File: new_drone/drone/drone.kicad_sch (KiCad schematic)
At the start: 29 parts, among them J1 Conn_01x06, SW1 SW_Push_Open, SW2 SW_Push_Open, U1 ESP32-WROOM-32, U2 MPU-6050, U4 BMP280, U5 MCP8063, U5 TPS63001, U6 MCP8063, U7 MCP8063, U8 MCP8063

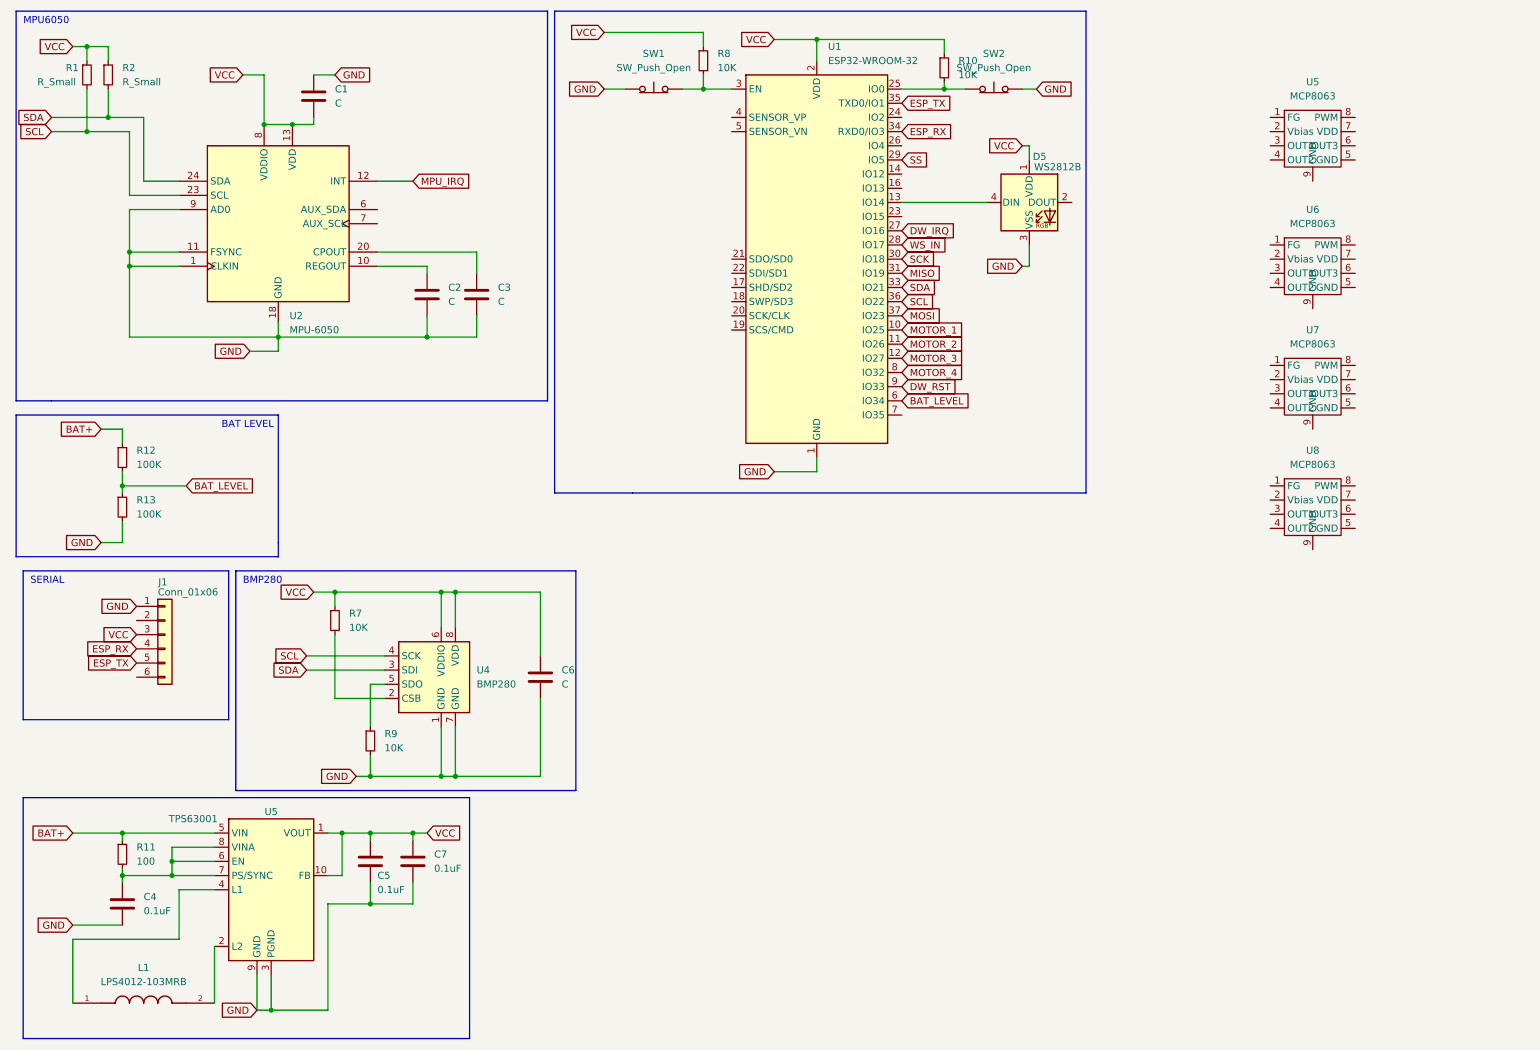
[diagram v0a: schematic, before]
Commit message: first wiring
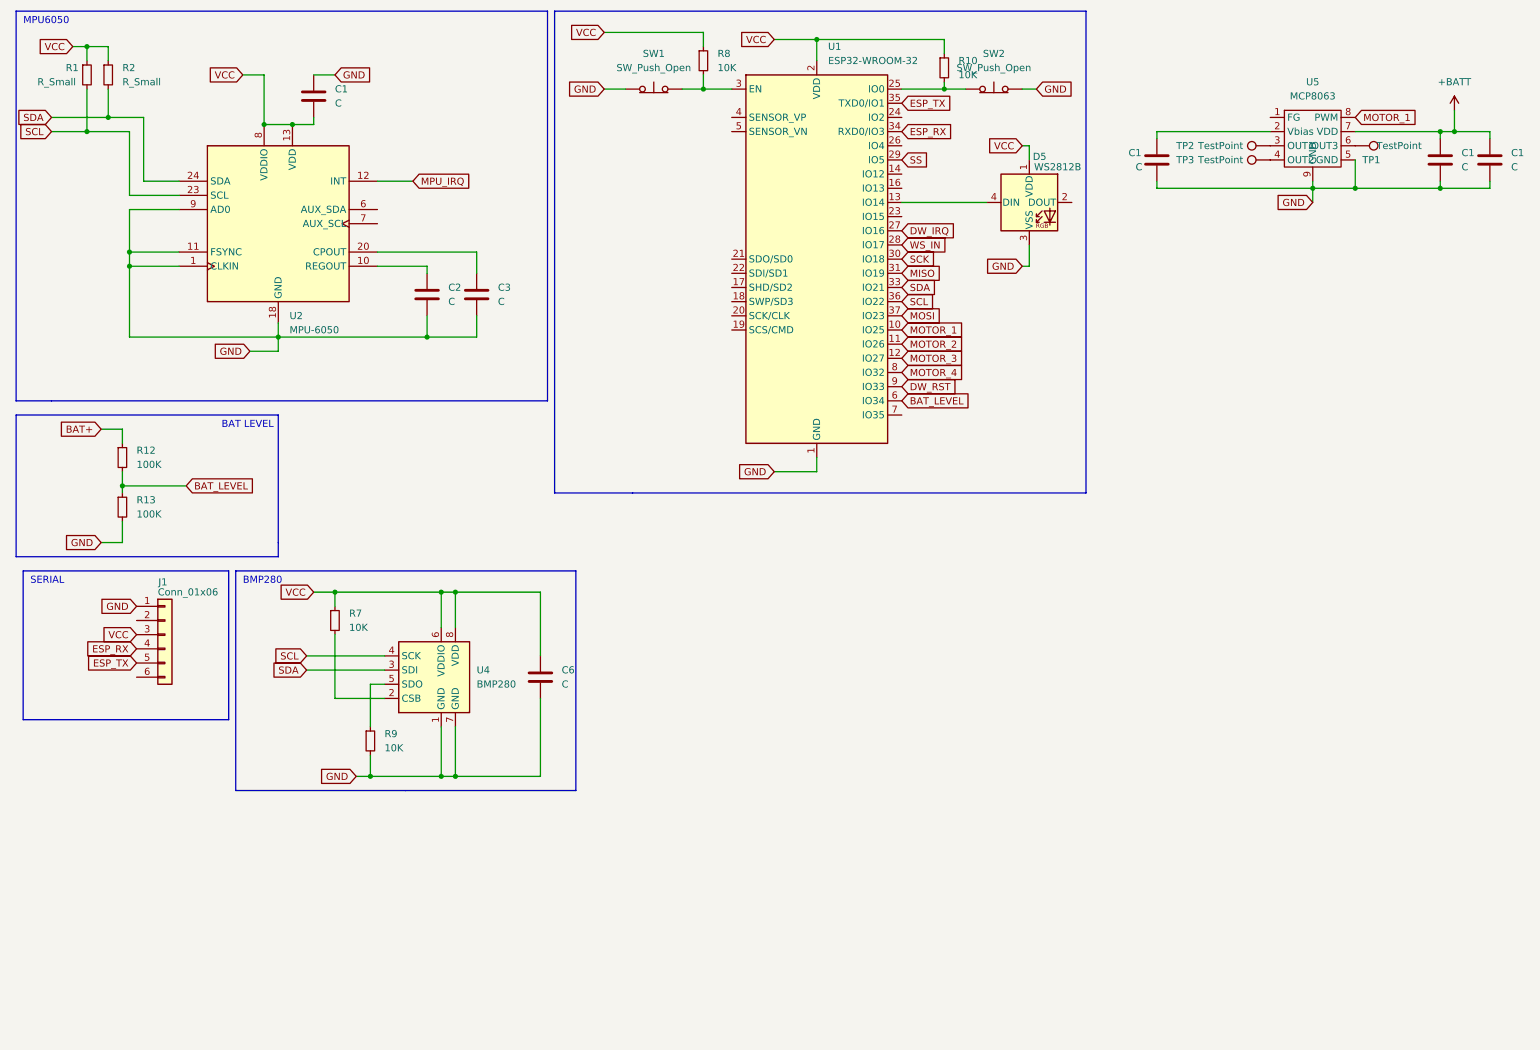
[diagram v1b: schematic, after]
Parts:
- removed C4, C5, C7: 0.1uF, Capacitor_SMD:C_0603_1608Metric, symbol Device:C
- removed L1: LPS4012-103MRB, LPS4012:IND_LPS4012-103MRB, symbol LPS4012:LPS4012-103MRB
- removed R11: 100, Resistor_SMD:R_0603_1608Metric, symbol Device:R_Small
- removed U5: TPS63001, Package_SON:Texas_DRC0010J_ThermalVias, symbol Regulator_Switching:TPS63000
- removed U6, U7, U8: MCP8063, Package_DFN_QFN:DFN-8-1EP_4x4mm_P0.8mm_EP2.5x3.6mm, symbol MCP8063:MCP8063
- added C1 (x3): C, Capacitor_SMD:C_0603_1608Metric, symbol Device:C
- added TP1, TP2, TP3: TestPoint, TestPoint:TestPoint_Pad_3.0x3.0mm, symbol Connector:TestPoint
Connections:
- net GND: now also U5.5 (GND), U5.9 (GND), C1.2, C1.2, C1.2
- net MOTOR_1: now also U5.8 (PWM)
- net at U5.2 (Vbias): now also C1.1
- net at U5.3 (OUT1): now also TP2.1
- net at U5.4 (OUT2): now also TP3.1
- net at U5.6 (OUT3): now also TP1.1
- net +BATT: now reaches U5.7 (VDD)
- net +BATT: now also C1.1, C1.1
